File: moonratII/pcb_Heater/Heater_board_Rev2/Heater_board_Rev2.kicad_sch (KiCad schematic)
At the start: 52 parts, among them J1 Barrel_Jack_Switch_SMT, J10 Conn_02x05_Odd_Even, J11 Screw_Terminal_01x02, J2 HS96L03W2C03_0.96_Oled, J5 Conn_02x05_Odd_Even, J6 Screw_Terminal_01x06, J9 Screw_Terminal_01x06, Q1 IRF540N, Q2 BSS138, SW1 6mm 2 Pin Tact NO Breadboard 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, SW2 6mm 2 Pin Tact NO Breadboard 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, SW3 6mm 2 Pin Tact NO Breadboard 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, U1 TMP36GRTZ-REEL7

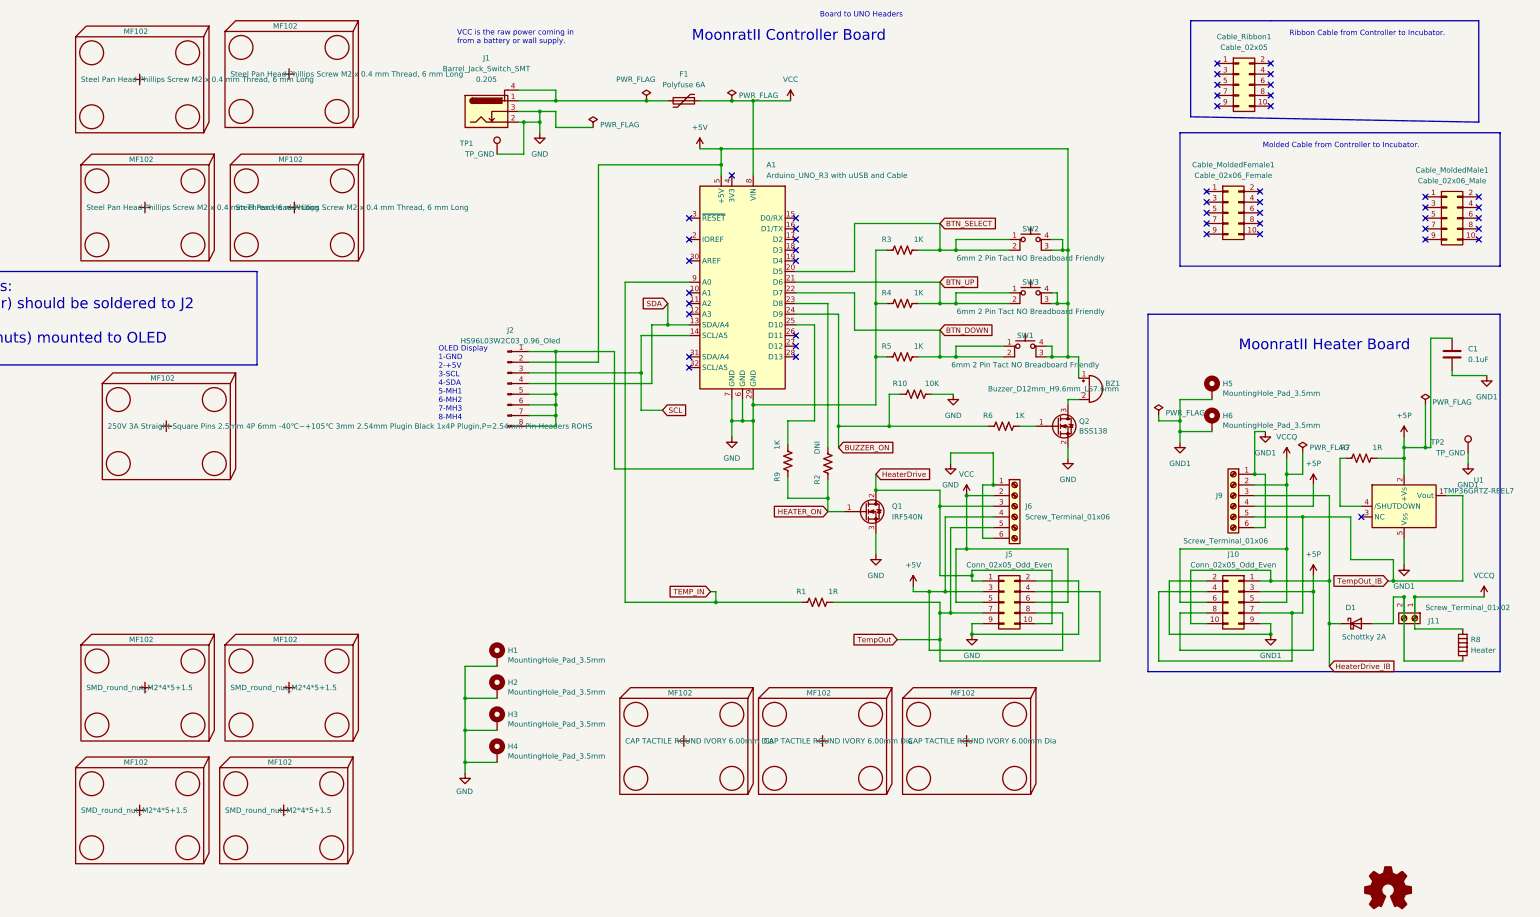
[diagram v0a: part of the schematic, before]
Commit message: Deleted controller from heater board Schematic and PCB files. Deleted proxy from Assy_Enclosure_Rev2_PWA.FCStd file.
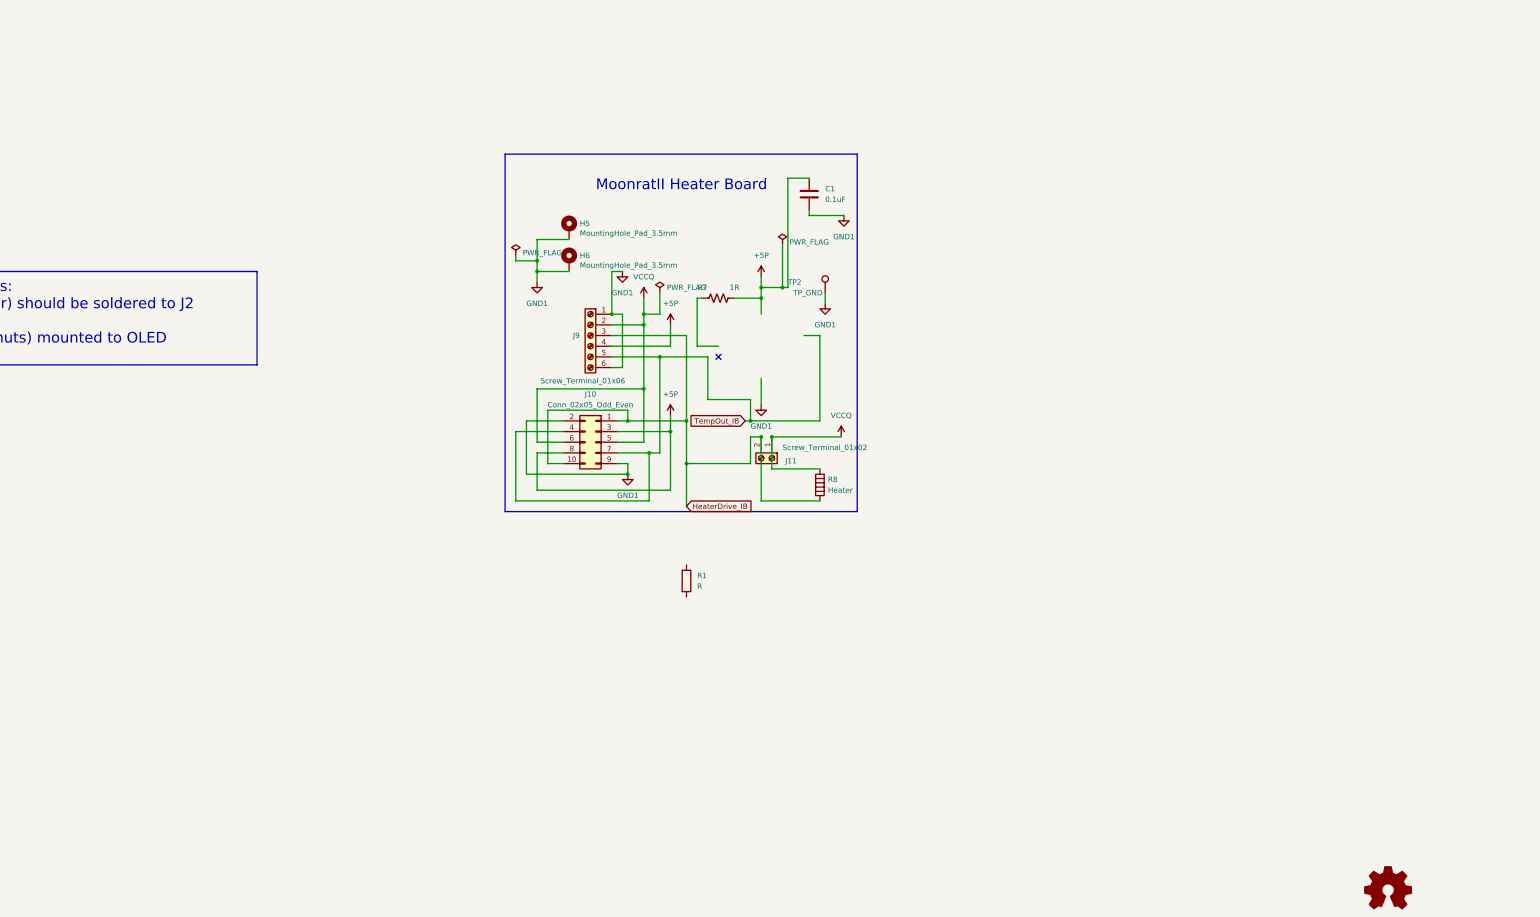
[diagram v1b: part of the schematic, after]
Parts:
- removed A1: Arduino_UNO_R3 with uUSB and Cable, GeneralPurposeAlarmDevicePCB:Arduino_UNO_R3_NoMountingHoles3D_Text_Top_&_Bottom, symbol MCU_Module:Arduino_UNO_R3
- removed BZ1: Buzzer_D12mm_H9.6mm_LS7.6mm, GeneralPurposeAlarmDevicePCB:Buzzer_12.2mm_9.7mm_7.62mm, symbol GPAD_SCH_LIB:Buzzer_Adafruit_P1536A
- removed Cable_MoldedFemale1: Cable_02x06_Female, symbol Connector_Generic:Conn_02x05_Odd_Even
- removed Cable_MoldedMale1: Cable_02x06_Male, symbol Connector_Generic:Conn_02x05_Odd_Even
- removed Cable_Ribbon1: Cable_02x05, symbol Connector_Generic:Conn_02x05_Odd_Even
- removed D1: Schottky 2A, Diode_SMD:D_SMB, symbol Device:D_Schottky
- removed F1: Polyfuse 6A, GeneralPurposeAlarmDevicePCB:Fuse_BSMD_1812, symbol Device:Polyfuse
- removed H1, H2, H3, H4: MountingHole_Pad_3.5mm, GeneralPurposeAlarmDevicePCB:MountingHole_3.5mm_Pad_Via, symbol GPAD_SCH_LIB:MountingHole_Pad_3.5mm
- removed J1: Barrel_Jack_Switch_SMT, GeneralPurposeAlarmDevicePCB:BarrelJack_CLIFF_FC681465S_SMT_Horizontal, symbol GPAD_SCH_LIB:Barrel_Jack_Switch_SMT
- removed J2: HS96L03W2C03_0.96_Oled, GeneralPurposeAlarmDevicePCB:OLED_HS96L03W2C03_0.96_WithNuts, symbol Connector:Conn_01x08_Pin
- removed J5: Conn_02x05_Odd_Even, Connector_IDC:IDC-Header_2x05_P2.54mm_Vertical, symbol Connector_Generic:Conn_02x05_Odd_Even
- removed J6: Screw_Terminal_01x06, GeneralPurposeAlarmDevicePCB:1x6P 20A -40℃~+105℃ 300V Green 12~30 Straight pin 5.08mm 2.5 1 6 Plugin,P=5.08mm Screw ter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, symbol Connector:Screw_Terminal_01x06
- removed MF102 (x4): SMD_round_nut_M2*4*5+1.5, TH162050CTJ, symbol GPAD_SCH_LIB:ENCLOSURE_GPAD_VER1
- removed MF102 (x3): CAP TACTILE ROUND IVORY 6.00mm Dia, B32-2000, symbol GPAD_SCH_LIB:ENCLOSURE_GPAD_VER1
- removed MF102 (x4): Steel Pan Head Phillips Screw M2 x 0.4 mm Thread,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, symbol GPAD_SCH_LIB:ENCLOSURE_GPAD_VER1
- removed MF102: 250V 3A Straight Square Pins 2.5mm 4P 6mm -40℃~+1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, PZ254V-11-04P, symbol GPAD_SCH_LIB:ENCLOSURE_GPAD_VER1
- removed Q1: IRF540N, Package_TO_SOT_THT:TO-220-3_Horizontal_TabDown, symbol Transistor_FET:IRF540N
- removed Q2: BSS138, Package_TO_SOT_SMD:SOT-23, symbol Transistor_FET:BSS138
- removed R1: 1R, Resistor_SMD:R_0603_1608Metric_Pad0.98x0.95mm_HandSolder, symbol Device:R_US
- removed R10: 10K, Resistor_SMD:R_0603_1608Metric_Pad0.98x0.95mm_HandSolder, symbol Device:R_US
- removed R2: DNI, Resistor_SMD:R_0603_1608Metric_Pad0.98x0.95mm_HandSolder, symbol Device:R_US
- removed R3, R4, R5, R6, R9: 1K, Resistor_SMD:R_0603_1608Metric_Pad0.98x0.95mm_HandSolder, symbol Device:R_US
- removed SW1, SW2, SW3: 6mm 2 Pin Tact NO Breadboard Friendly, GeneralPurposeAlarmDevicePCB:Switch_Tactile_THT_6x6mm, symbol Switch:SW_MEC_5E
- removed TP1: TP_GND, TestPoint:TestPoint_Loop_D2.54mm_Drill1.5mm_Beaded, symbol Connector:TestPoint
- removed U1: TMP36GRTZ-REEL7, Package_TO_SOT_SMD:SOT-23-5, symbol GPAD_SCH_LIB:TMP36GRTZ-REEL7
- added R1: R, symbol Device:R
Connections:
- net HeaterDrive_IB: now also J11.2 (Pin_2), R8.1
- no-connect marks 48 -> 1
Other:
- note removed: "Board to UNO Headers"
- note removed: "Molded Cable from Controller to Incubator."
- note removed: "MoonratII Controller Board"
- note removed: "OLED Display 1-GND 2-+5V 3-SCL 4-SDA 5-MH1 6-MH2 7-MH3 8-MH4"
- note removed: "Ribbon Cable from Controller to Incubator."
- note removed: "VCC is the raw power coming in from a battery or wall supply."
- moved on the sheet: C1, H5, H6, J10, J11, J9, R7, R8, TP2

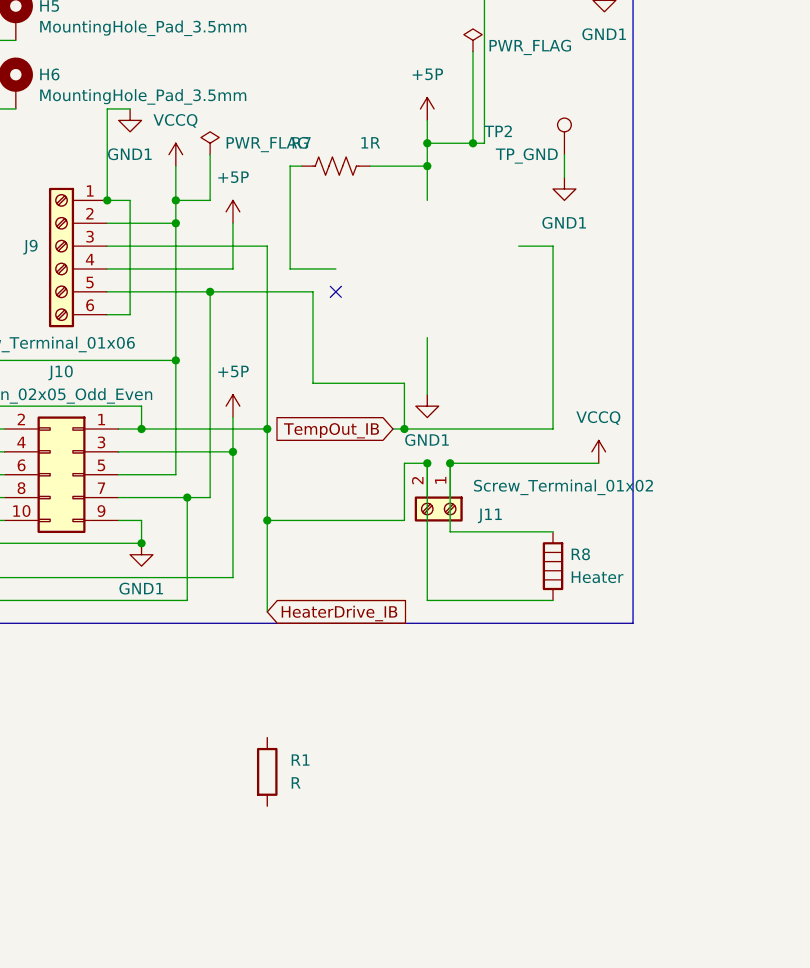
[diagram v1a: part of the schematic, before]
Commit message: Added a 4.7 pull up resistor to heater board.
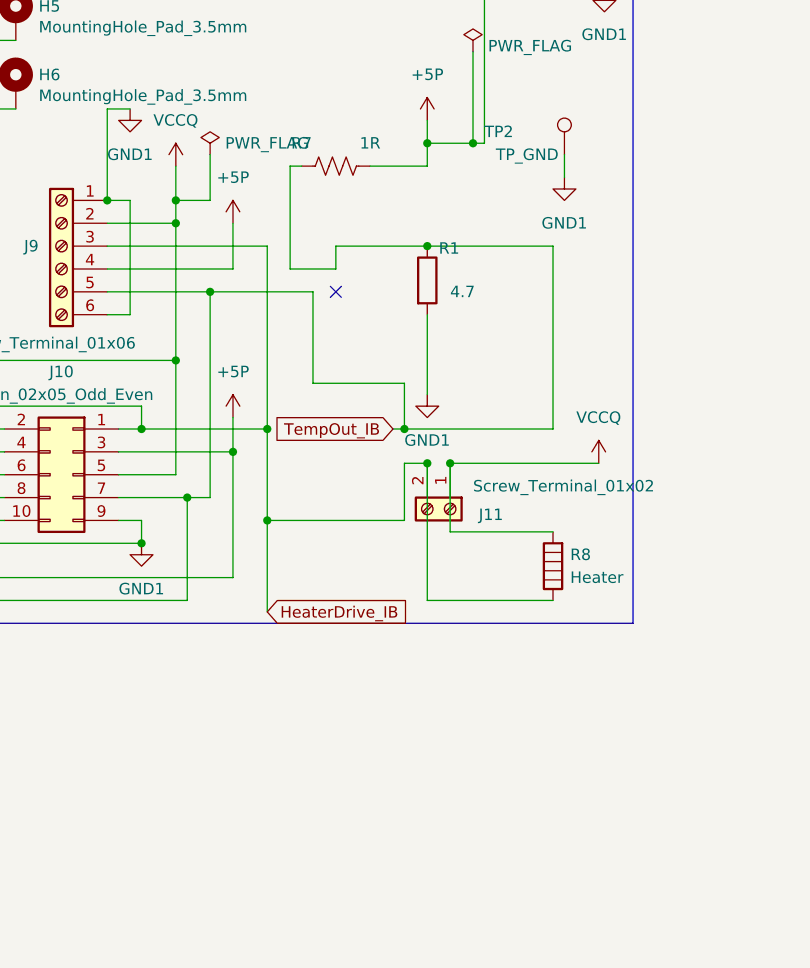
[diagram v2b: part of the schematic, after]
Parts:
- R1: value R -> 4.7; footprint (none) -> /Users/melanielaporte/Desktop/4.7ohm C3473875 datasheet
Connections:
- net GND1: now also R1.2
- net TempOut_IB: now also R1.1, R7.1
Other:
- moved on the sheet: R1
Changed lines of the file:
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@@
 	)
 	(junction
-		(at 234.95 102.87)
-		(diameter 0)
-		(color 0 0 0 0)
-	)
-	(junction
 		(at 203.2 144.78)
 		(diameter 0)
@@
 		(color 0 0 0 0)
 	)
+	(junction
+		(at 234.95 111.76)
+		(diameter 0)
+		(color 0 0 0 0)
+	)
 	(no_connect
 		(at 224.79 116.84)
@@
 	(wire
 		(pts
-			(xy 234.95 102.87) (xy 234.95 106.68)
-		)
-		(stroke
-			(width 0)
-			(type default)
-		)
-	)
-	(wire
-		(pts
 			(xy 203.2 142.24) (xy 203.2 144.78)
 		)
@@
 		)
 	)
-	(wire
-		(pts
-			(xy 248.92 111.76) (xy 245.11 111.76)
-		)
-		(stroke
-			(width 0)
-			(type default)
-		)
-	)
 	(polyline
 		(pts
@@
 	(wire
 		(pts
-			(xy 234.95 121.92) (xy 234.95 128.27)
+			(xy 234.95 119.38) (xy 234.95 128.27)
 		)
 		(stroke
@@
 	(wire
 		(pts
+			(xy 224.79 111.76) (xy 234.95 111.76)
+		)
+		(stroke
+			(width 0)
+			(type default)
+		)
+	)
+	(wire
+		(pts
 			(xy 189.23 88.9) (xy 181.61 88.9)
 		)
@@
 	(wire
 		(pts
+			(xy 234.95 111.76) (xy 248.92 111.76)
+		)
+		(stroke
+			(width 0)
+			(type default)
+		)
+	)
+	(wire
+		(pts
+			(xy 224.79 114.3) (xy 224.79 111.76)
+		)
+		(stroke
+			(width 0)
+			(type default)
+		)
+	)
+	(wire
+		(pts
 			(xy 231.14 132.08) (xy 232.41 132.08)
 		)
@@
 	(symbol
 		(lib_id "Device:R")
-		(at 217.17 170.18 0)
+		(at 234.95 115.57 0)
 		(unit 1)
 		(exclude_from_sim no)
@@
 		(on_board yes)
 		(dnp no)
-		(fields_autoplaced yes)
 		(property "Reference" "R1"
-			(at 219.71 168.9099 0)
+			(at 236.22 112.014 0)
 			(effects
 				(font
@@
 			)
 		)
-		(property "Value" "R"
-			(at 219.71 171.4499 0)
+		(property "Value" "4.7"
+			(at 237.49 116.8399 0)
 			(effects
 				(font
@@
 			)
 		)
-		(property "Footprint" ""
-			(at 215.392 170.18 90)
+		(property "Footprint" "/Users/melanielaporte/Desktop/4.7ohm C3473875 datasheet"
+			(at 233.172 115.57 90)
 			(effects
 				(font
@@
 		)
 		(property "Datasheet" "~"
-			(at 217.17 170.18 0)
+			(at 234.95 115.57 0)
 			(effects
 				(font
@@
 		)
 		(property "Description" "Resistor"
-			(at 217.17 170.18 0)
+			(at 234.95 115.57 0)
 			(effects
 				(font
